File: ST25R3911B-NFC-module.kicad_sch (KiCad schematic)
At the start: 46 parts, among them J1 USB_C_Receptacle_USB2.0_16P, SW2 SW_Push, SW3 SW_Push, U1 ST25R3911B-AQF, U2 AP1117-33, U3 W25Q128JVS, U4 RP2040, Y1 Crystal_GND24

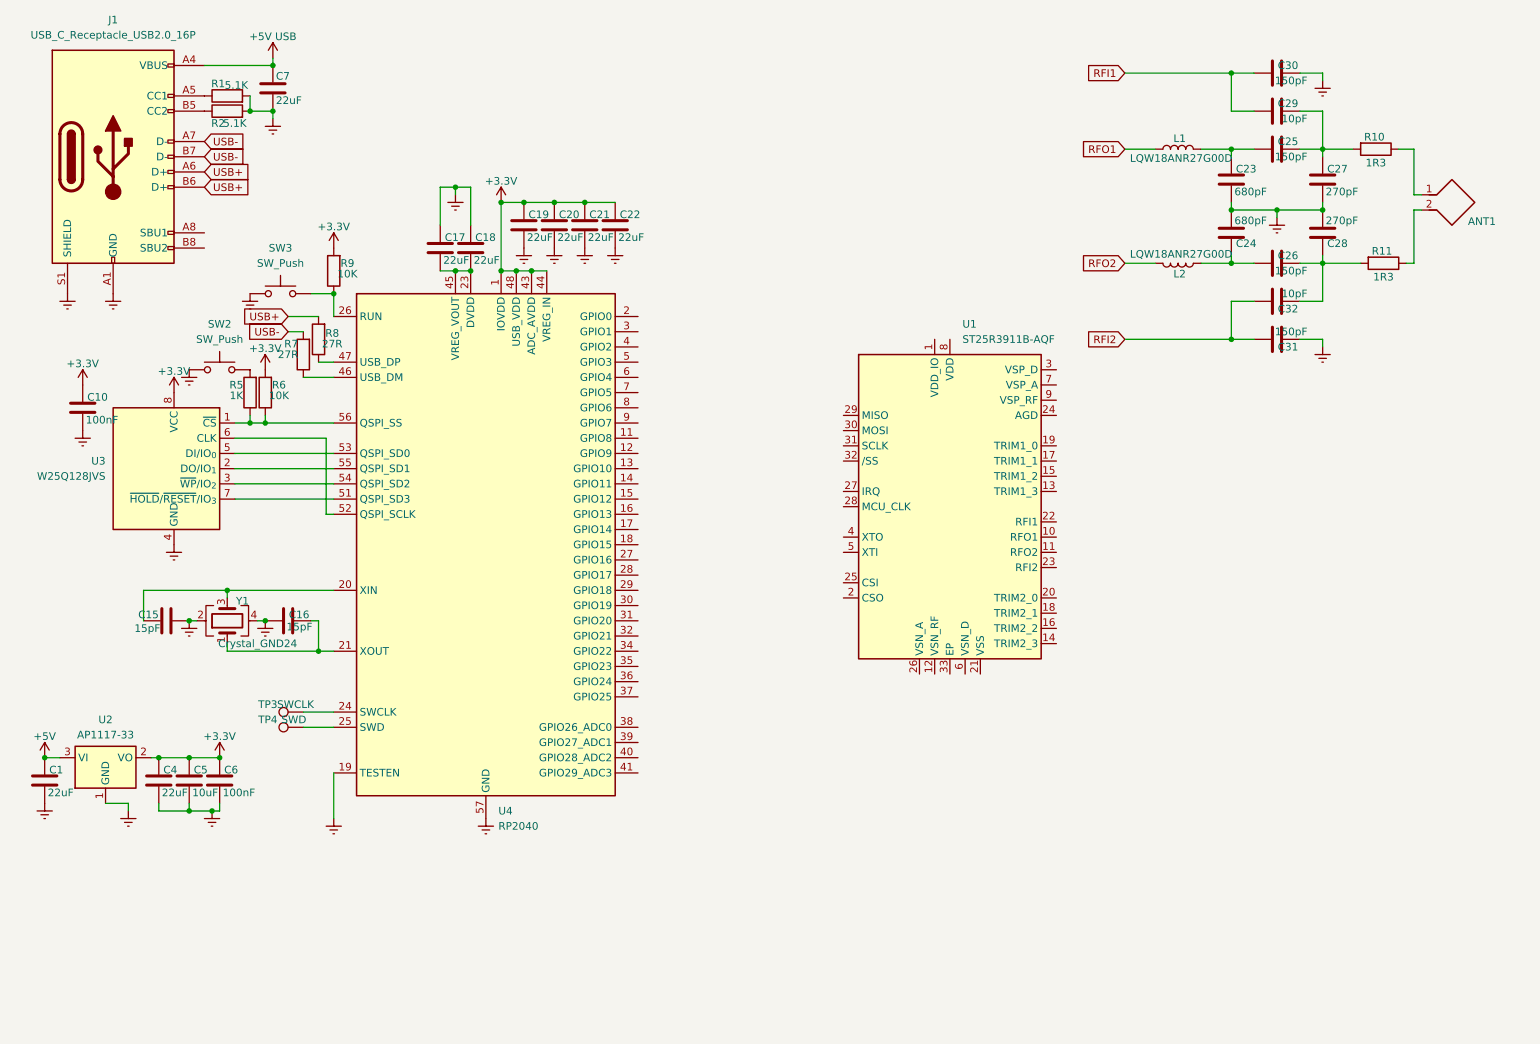
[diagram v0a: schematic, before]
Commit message: схему вроде сделал, надо только понять как вообще адекватно, а главное симметрично мне провести к антенне всё что надобно
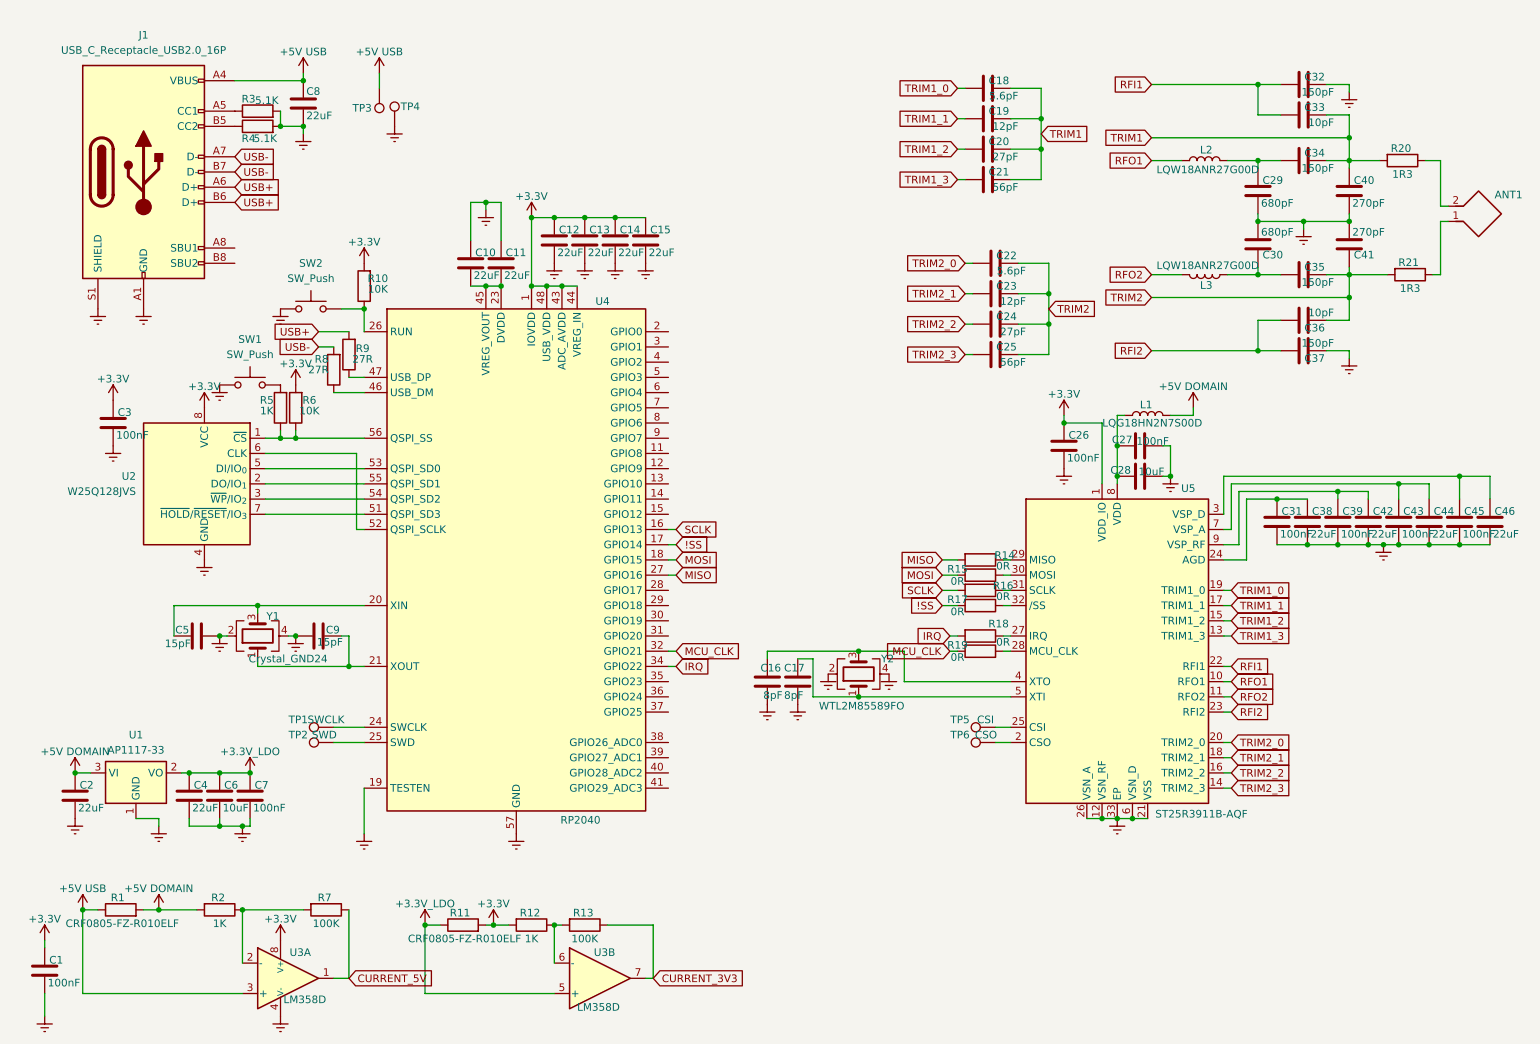
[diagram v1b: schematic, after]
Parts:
- added C1, C26, C27, C31, C39, C43, C45: 100nF, Capacitor_SMD:C_0402_1005Metric, symbol Device:C
- added C16, C17: 8pF, Capacitor_SMD:C_0402_1005Metric, symbol Device:C
- added C18, C22: 5.6pF, Capacitor_SMD:C_0402_1005Metric, symbol Device:C
- added C19, C23: 12pF, Capacitor_SMD:C_0402_1005Metric, symbol Device:C
- added C20, C24: 27pF, Capacitor_SMD:C_0402_1005Metric, symbol Device:C
- added C21, C25: 56pF, Capacitor_SMD:C_0402_1005Metric, symbol Device:C
- added C28: 10uF, Capacitor_SMD:C_0402_1005Metric, symbol Device:C
- added C38, C42, C44, C46: 22uF, Capacitor_SMD:C_0402_1005Metric, symbol Device:C
- added L1: LQG18HN2N7S00D, Inductor_SMD:L_0603_1608Metric, symbol Device:L
- added R1: CRF0805-FZ-R010ELF, PCM_Resistor_SMD_AKL:R_0805_2012Metric_Pad1.15x1.40mm, symbol Device:R
- added R11: CRF0805-FZ-R010ELF, PCM_Resistor_SMD_AKL:R_0805_2012Metric, symbol Device:R
- added R12, R2: 1K, PCM_Resistor_SMD_AKL:R_0402_1005Metric, symbol Device:R
- added R13, R7: 100K, PCM_Resistor_SMD_AKL:R_0402_1005Metric, symbol Device:R
- added R14, R15, R16, R17, R18, R19: 0R, PCM_Resistor_SMD_AKL:R_0402_1005Metric, symbol Device:R
- added TP3, TP4: ~, TestPoint:TestPoint_Pad_1.5x1.5mm, symbol Connector:TestPoint
- added TP5: CSI, TestPoint:TestPoint_Pad_D1.0mm, symbol Connector:TestPoint
- added TP6: CSO, TestPoint:TestPoint_Pad_D1.0mm, symbol Connector:TestPoint
- added U3: LM358D, PCM_Package_SO_AKL:SO-8_3.9x4.9mm_P1.27mm, symbol PCM_Amplifier_Operational_AKL:LM358D
- added Y2: WTL2M85589FO, Crystal:Crystal_SMD_2520-4Pin_2.5x2.0mm, symbol Device:Crystal_GND24
- renumbered C17 to C10, C18 to C11, C19 to C12, C20 to C13, C21 to C14, C22 to C15, C1 to C2, C23 to C29, C10 to C3, C24 to C30, C30 to C32, C29 to C33, C25 to C34, C26 to C35, C32 to C36, C31 to C37, C27 to C40, C28 to C41, C15 to C5, C5 to C6, C6 to C7, C7 to C8, C16 to C9, L1 to L2, L2 to L3, R9 to R10, R10 to R20, R11 to R21, R1 to R3, R2 to R4, R7 to R8, R8 to R9, SW2 to SW1, SW3 to SW2, TP3 to TP1, TP4 to TP2, U2 to U1, U3 to U2, U1 to U5
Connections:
- net +3.3V: now also U5.1 (VDD_IO), C1.1, C26.1, R11.2, R12.2, U3.8 (V+); no longer C4.1, C6.1, C7.1, U1.2 (VO)
- net +5V USB: now also R1.1, TP3.1, U3.3 (+)
- net Earth: now also U5.12 (VSN_RF), U5.21 (VSS), U5.26 (VSN_A), U5.33 (EP), U5.6 (VSN_D), C1.2, C16.1, C17.2, C26.2, C27.2, C28.2, C31.2, C38.2, C39.2, C42.2, C43.2, C44.2, C45.2, C46.2, TP4.1, U3.4 (V-), Y2.2, Y2.4
- net RFI1: now also U5.22 (RFI1)
- net RFI2: now also U5.23 (RFI2)
- net RFO1: now also U5.10 (RFO1)
- net RFO2: now also U5.11 (RFO2)
- net TRIM2: now reaches C35.2, C36.2, C41.1, R21.2
- net TRIM2: now also C22.2, C23.2, C24.2, C25.2
- net TRIM1: now reaches C33.2, C34.2, C40.1, R20.2
- net TRIM1: now also C18.2, C19.2, C20.2, C21.2
- net SCLK: now reaches U4.16 (GPIO13)
- net SCLK: now also R16.2
- net !SS: now reaches U4.17 (GPIO14)
- net !SS: now also R17.2
- net MOSI: now reaches U4.18 (GPIO15)
- net MOSI: now also R15.2
- net MISO: now reaches U4.27 (GPIO16)
- net MISO: now also R14.2
- net MCU_CLK: now reaches U4.32 (GPIO21)
- net MCU_CLK: now also R19.2
- net IRQ: now reaches U4.34 (GPIO22)
- net IRQ: now also R18.2
- net at R20.1: now also ANT1.2; no longer ANT1.1
- net at R21.1: now also ANT1.1; no longer ANT1.2
- net TRIM1_3: now reaches U5.13 (TRIM1_3)
- net TRIM1_3: now also C21.1
- net TRIM2_3: now reaches U5.14 (TRIM2_3)
- net TRIM2_3: now also C25.1
- net TRIM1_2: now reaches U5.15 (TRIM1_2)
- net TRIM1_2: now also C20.1
- net TRIM2_2: now reaches U5.16 (TRIM2_2)
- net TRIM2_2: now also C24.1
- net TRIM1_1: now reaches U5.17 (TRIM1_1)
- net TRIM1_1: now also C19.1
- net TRIM2_1: now reaches U5.18 (TRIM2_1)
- net TRIM2_1: now also C23.1
- net TRIM1_0: now reaches U5.19 (TRIM1_0)
- net TRIM1_0: now also C18.1
- net at U5.2 (CSO): now also TP6.1
- net TRIM2_0: now reaches U5.20 (TRIM2_0)
- net TRIM2_0: now also C22.1
- net at U5.24 (AGD): now also C31.1, C38.1
- net at U5.25 (CSI): now also TP5.1
- net at U5.27 (IRQ): now also R18.1
- net at U5.28 (MCU_CLK): now also R19.1
- net at U5.29 (MISO): now also R14.1
- net at U5.3 (VSP_D): now also C45.1, C46.1
- net at U5.30 (MOSI): now also R15.1
- net at U5.31 (SCLK): now also R16.1
- net at U5.32 (/SS): now also R17.1
- net at U5.4 (XTO): now also C16.2, Y2.3
- net at U5.5 (XTI): now also C17.1, Y2.1
- net at U5.7 (VSP_A): now also C43.1, C44.1
- net at U5.8 (VDD): now also C27.1, C28.1, L1.2
- net at U5.9 (VSP_RF): now also C39.1, C42.1
- net +5V renamed +5V DOMAIN
- net +5V DOMAIN: now also L1.1, R1.2, R2.2
- new net: R12.1, R13.2, U3.6 (-)
- new net: R2.1, R7.2, U3.2 (-)
- new net +3.3V_LDO: C4.1, C6.1, C7.1, R11.1, U1.2 (VO), U3.5 (+)
- new net CURRENT_3V3: R13.1, U3.7
- new net CURRENT_5V: R7.1, U3.1
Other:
- moved on the sheet: ANT1, C10, C11, C12, C13, C14, C15, C2, C29, C3, C30, C32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

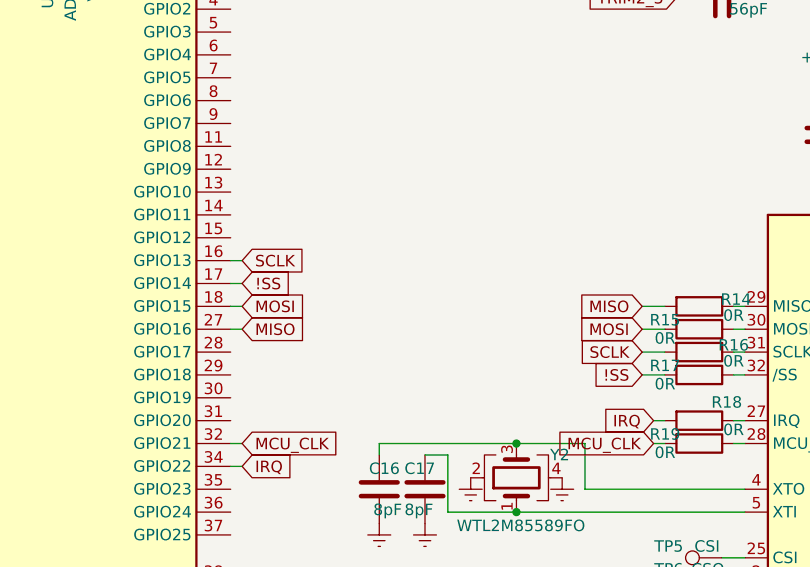
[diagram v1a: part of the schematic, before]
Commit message: rev0 готова
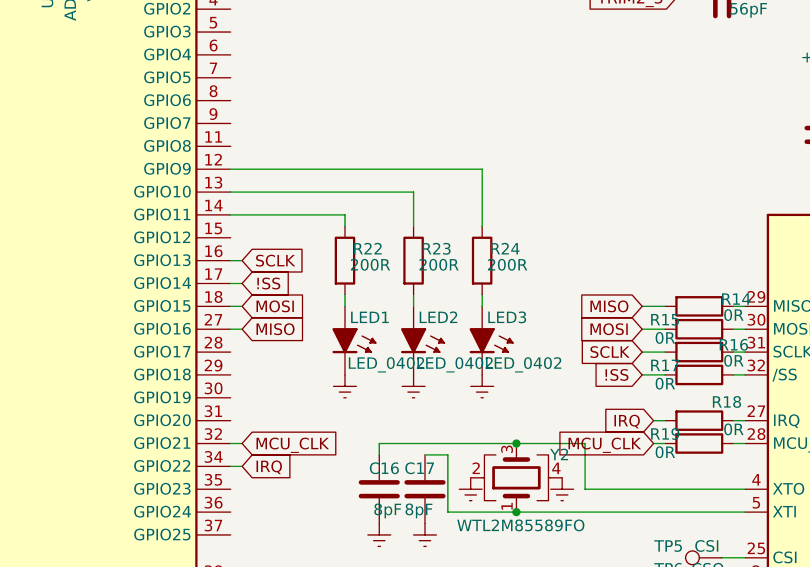
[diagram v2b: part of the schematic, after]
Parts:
- added LED1, LED2, LED3: LED_0402, LED_SMD:LED_0402_1005Metric, symbol PCM_LED_AKL:LED_0402
- added R22, R23, R24: 200R, PCM_Resistor_SMD_AKL:R_0402_1005Metric, symbol Device:R
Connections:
- net Earth: now also LED1.1 (K), LED2.1 (K), LED3.1 (K)
- net at U4.12 (GPIO9): now also R24.1
- net at U4.13 (GPIO10): now also R23.1
- net at U4.14 (GPIO11): now also R22.1
- new net: LED3.2 (A), R24.2
- new net: LED2.2 (A), R23.2
- new net: LED1.2 (A), R22.2
